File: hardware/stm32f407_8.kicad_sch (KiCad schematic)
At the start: 28 parts, among them J10 Conn_01x04, J8 GMSB0531112YEU, J9 Conn_01x04, SW3 SW TACT-SPST, U7 STM32F407VGT6, Y3 ABM8G-8.000MHZ-18-D2Y-T

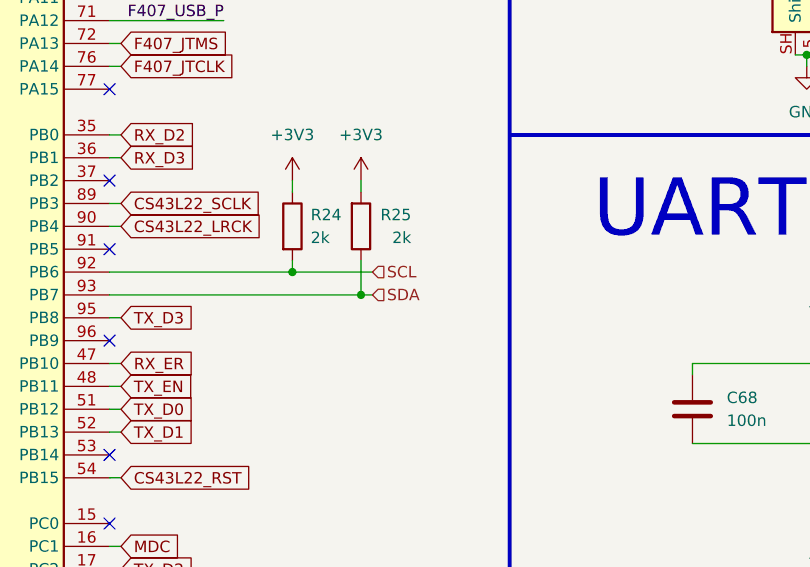
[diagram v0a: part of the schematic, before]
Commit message: Fix DRC errors
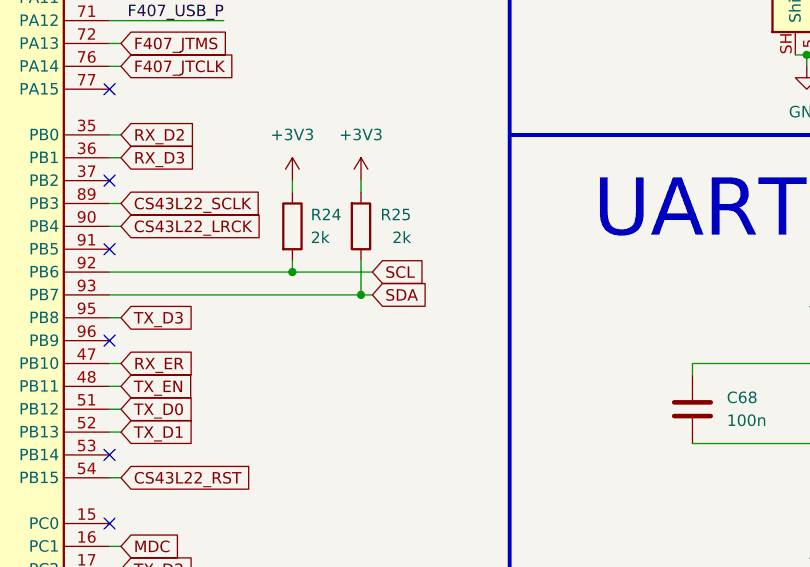
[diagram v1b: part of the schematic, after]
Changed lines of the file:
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@@
+		)
+	)
+	(global_label "SCL"
+		(shape input)
+		(at 160.02 109.22 0)
+		(fields_autoplaced yes)
+		(effects
+			(font
+				(size 1.27 1.27)
+			)
+			(justify left)
+		)
+		(property "Intersheetrefs" "${INTERSHEET_REFS}"
+			(at 166.5128 109.22 0)
+			(hide yes)
+			(show_name no)
+			(do_not_autoplace no)
+			(effects
+				(font
+					(size 1.27 1.27)
+				)
+				(justify left)
+			)
 		)
 	)
@@
 		)
 	)
+	(global_label "SDA"
+		(shape input)
+		(at 160.02 111.76 0)
+		(fields_autoplaced yes)
+		(effects
+			(font
+				(size 1.27 1.27)
+			)
+			(justify left)
+		)
+		(property "Intersheetrefs" "${INTERSHEET_REFS}"
+			(at 166.5733 111.76 0)
+			(hide yes)
+			(show_name no)
+			(do_not_autoplace no)
+			(effects
+				(font
+					(size 1.27 1.27)
+				)
+				(justify left)
+			)
+		)
+	)
 	(global_label "MIC_CLK"
 		(shape input)
@@
 		)
 	)
-	(hierarchical_label "SDA"
-		(shape input)
-		(at 160.02 111.76 0)
-		(effects
-			(font
-				(size 1.27 1.27)
-			)
-			(justify left)
-		)
-	)
-	(hierarchical_label "SCL"
-		(shape input)
-		(at 160.02 109.22 0)
-		(effects
-			(font
-				(size 1.27 1.27)
-			)
-			(justify left)
-		)
-	)
